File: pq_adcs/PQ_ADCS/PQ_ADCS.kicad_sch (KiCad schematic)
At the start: 51 parts, among them J1 CES-110-02-L-S, J10 Pico-Clasp_01x09, J11 Pico-Clasp_01x15, J12 CES-102-02-L-S, J2 CES-110-02-L-S, J3 CES-110-02-L-S, J4 CES-110-02-L-S, J5 Pico-Clasp_01x03, J6 Pico-Clasp_01x10, J7 Pico-Clasp_01x10, J8 Pico-Clasp_01x10, J9 Pico-Clasp_01x10, U1 LPV542, U2 LPV542, U3 LPV542, U4 IIM-42652, U5 BD2606MVV, U6 TMUX1108RSVR, U7 MMC5983MA

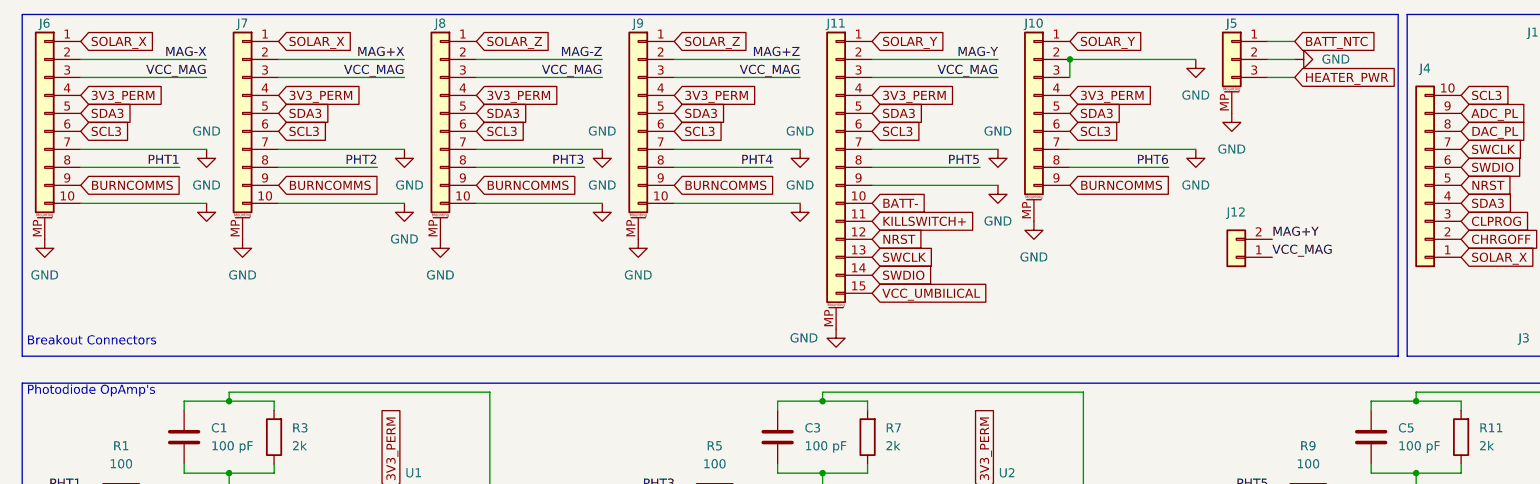
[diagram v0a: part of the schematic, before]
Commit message: fabrication
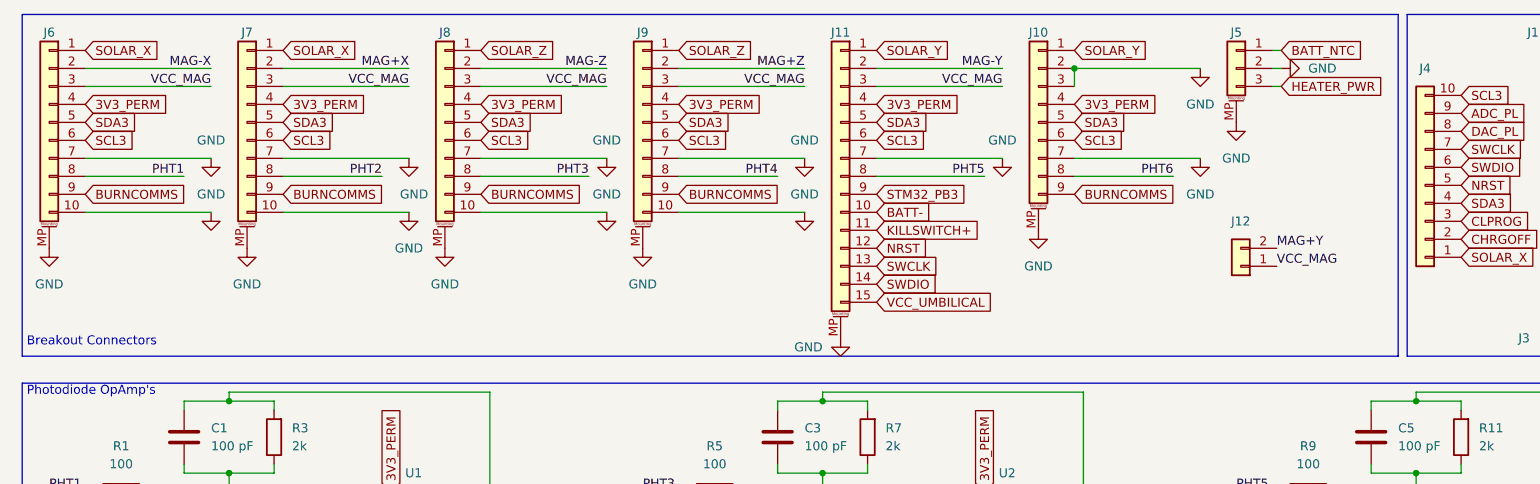
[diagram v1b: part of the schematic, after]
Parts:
- Annotation1: footprint -nsl_symbols:Bike -> symbols-nsl:Bike
- Annotation2: footprint -nsl_symbols:Bridgemaker -> symbols-nsl:Bridgemaker
- J1, J2, J3, J4: footprint -nsl_connector:SLW-110-01 -> connector-nsl:SLW-110-01
- J10: footprint -nsl_connector:Picoclasp09 -> connector-nsl:Picoclasp09
- J11: footprint -nsl_connector:Picoclasp15 -> connector-nsl:Picoclasp15
- J12: footprint -nsl_connector:CES-102-02 -> connector-nsl:CES-102-02
- J5: footprint -nsl_connector:Picoclasp03 -> connector-nsl:Picoclasp03
- J6, J7, J8, J9: footprint -nsl_connector:Picoclasp10 -> connector-nsl:Picoclasp10
- U2, U3: footprint -nsl_miscellaneous:TI_X1SON-8_3x3mm -> miscelaneous-nsl:TI_X1SON-8_3x3mm
- U6: footprint -nsl_miscellaneous:UQFN-16_1.8x2.6_Pitch0.4mm -> miscelaneous-nsl:UQFN-16_1.8x2.6_Pitch0.4mm
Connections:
- net GND: no longer J11.9
- net STM32_PB3: now also J11.9
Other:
- moved on the sheet: J10, J11, J12, J5, J6, J7, J8, J9
